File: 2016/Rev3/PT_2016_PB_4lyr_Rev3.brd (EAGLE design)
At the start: 155.7 x 202.7 mm, 166 parts, among them Q1 MOSFET-NCHANNELFDD8780, Q12 2N7002, Q2 MMBT2222A, Q3 MOSFET-NCHANNELFDD8780, Q4 MMBT2222A

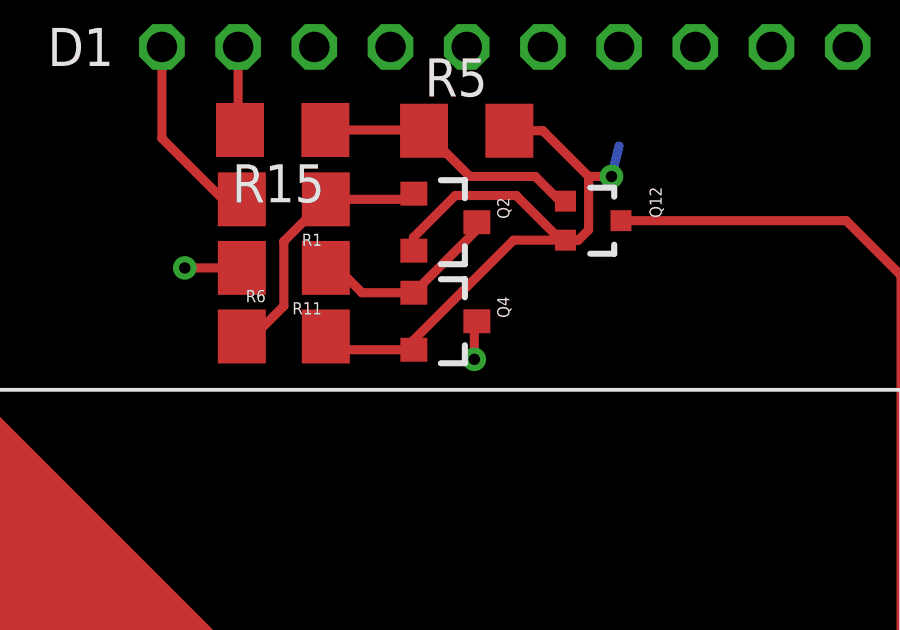
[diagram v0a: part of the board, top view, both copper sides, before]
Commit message: Fixed some routing
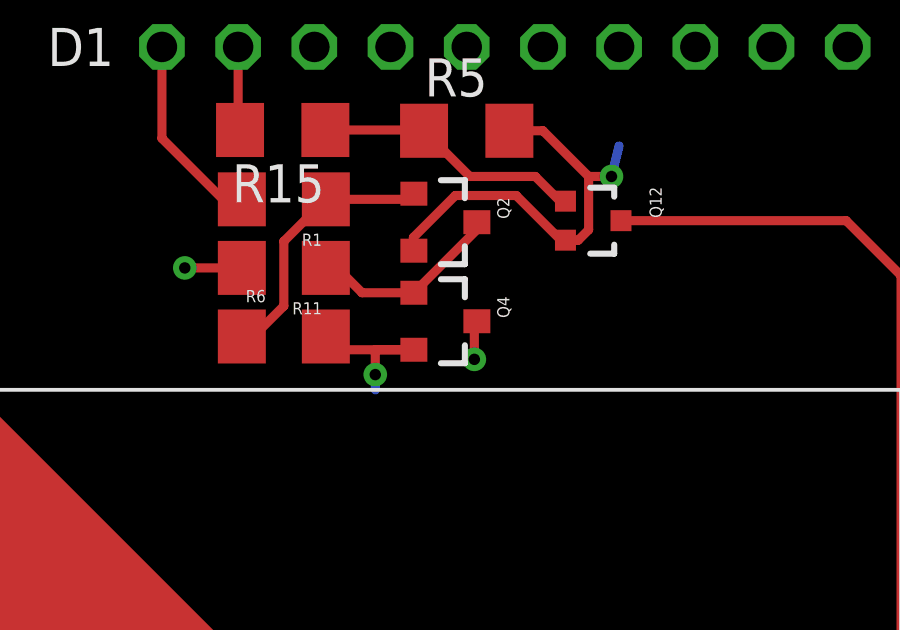
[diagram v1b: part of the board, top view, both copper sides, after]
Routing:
- net GND: track 213.0 -> 209.0 mm, vias 50 -> 51
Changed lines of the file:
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@@
 <contactref element="R6" pad="2"/>
 <wire x1="135.258" y1="143.764" x2="135.7" y2="143.322" width="0.3048" layer="1"/>
-<wire x1="135.7" y1="143.322" x2="138.192" y2="143.322" width="0.3048" layer="1"/>
 <wire x1="47.498" y1="150.746" x2="47.498" y2="150.876" width="0.3048" layer="1"/>
 <wire x1="47.498" y1="150.876" x2="47.752" y2="151.13" width="0.3048" layer="1"/>
@@
 <wire x1="143.6728" y1="146.9748" x2="143.2454" y2="146.9748" width="0.3048" layer="1"/>
 <wire x1="138.192" y1="143.322" x2="138.176" y2="143.338" width="0.3048" layer="1"/>
-<wire x1="138.176" y1="143.338" x2="138.176" y2="143.637" width="0.3048" layer="1"/>
-<wire x1="138.176" y1="143.637" x2="141.5138" y2="146.9748" width="0.3048" layer="1"/>
-<wire x1="141.5138" y1="146.9748" x2="143.0932" y2="146.9748" width="0.3048" layer="1"/>
 <wire x1="138.192" y1="146.624" x2="138.176" y2="146.64" width="0.3048" layer="1"/>
 <wire x1="138.176" y1="146.64" x2="138.176" y2="147.066" width="0.3048" layer="1"/>
@@
 <via x="144.78" y="149.098" extent="1-16" drill="0.381"/>
 <wire x1="144.78" y1="149.098" x2="145.034" y2="150.114" width="0.3048" layer="16"/>
+<wire x1="138.192" y1="143.322" x2="135.7" y2="143.322" width="0.3048" layer="1"/>
+<wire x1="138.192" y1="143.322" x2="136.906" y2="143.322" width="0.3048" layer="1"/>
+<wire x1="136.906" y1="143.322" x2="136.906" y2="142.494" width="0.3048" layer="1"/>
+<via x="136.906" y="142.494" extent="1-16" drill="0.381"/>
+<wire x1="136.906" y1="142.494" x2="136.906" y2="141.986" width="0.3048" layer="16"/>
 </signal>
 <signal name="V_BATT">
